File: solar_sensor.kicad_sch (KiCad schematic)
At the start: 4 parts

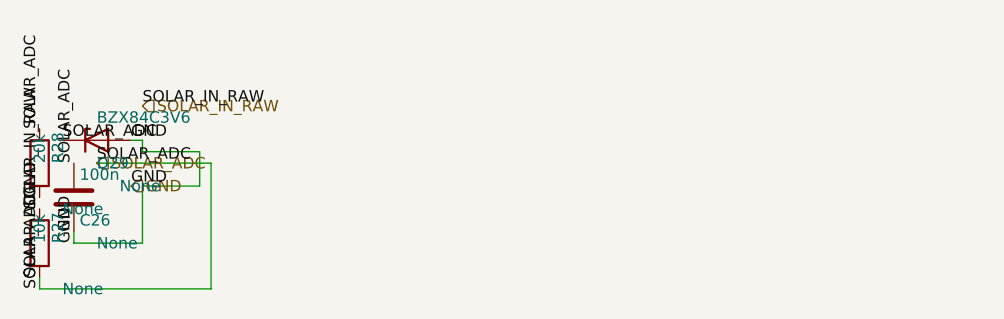
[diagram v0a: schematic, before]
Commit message: tests_fix
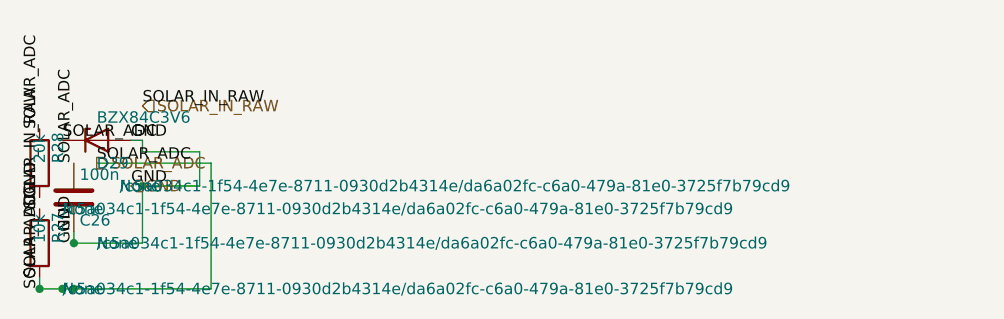
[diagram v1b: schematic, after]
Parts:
- C26, D29, R27, R28: hierarchy_path (none) -> /c5a034c1-1f54-4e7e-8711-0930d2b4314e/da6a02fc-c6a0-479a-81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
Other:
- title: (none) -> climate_control_niva_travel
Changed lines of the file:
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@@
 	(generator_version "9.0")
 	(paper "A4")
+	(title_block
+		(title "climate_control_niva_travel")
+	)
 	(symbol
 		(lib_id "Device:C")
@@
 			)
 		)
+		(property "hierarchy_path" "/c5a034c1-1f54-4e7e-8711-0930d2b4314e/da6a02fc-c6a0-479a-81e0-3725f7b79cd9"
+			(at 21.59 22.8599 0)
+			(effects
+				(font
+					(size 1.27 1.27)
+				)
+				(justify left)
+			)
+		)
 		(pin "1"
 		)
@@
 		)
 		(instances
-			(project "Untitled"
-				(path "/52be233a-28af-41aa-bdf8-43828795fcb1"
+			(project "climate_control_niva_travel"
+				(path "/c5a034c1-1f54-4e7e-8711-0930d2b4314e/da6a02fc-c6a0-479a-81e0-3725f7b79cd9"
 					(reference "C26")
 					(unit 1)
@@
 			)
 		)
+		(property "hierarchy_path" "/c5a034c1-1f54-4e7e-8711-0930d2b4314e/da6a02fc-c6a0-479a-81e0-3725f7b79cd9"
+			(at 17.78 27.9399 0)
+			(effects
+				(font
+					(size 1.27 1.27)
+				)
+				(justify left)
+			)
+		)
 		(pin "1"
 		)
@@
 		)
 		(instances
-			(project "Untitled"
-				(path "/52be233a-28af-41aa-bdf8-43828795fcb1"
-					(reference "R27")
+			(project "climate_control_niva_travel"
+				(path "/c5a034c1-1f54-4e7e-8711-0930d2b4314e/da6a02fc-c6a0-479a-81e0-3725f7b79cd9"
+					(reference "R43")
 					(unit 1)
 				)
@@
 			)
 		)
+		(property "hierarchy_path" "/c5a034c1-1f54-4e7e-8711-0930d2b4314e/da6a02fc-c6a0-479a-81e0-3725f7b79cd9"
+			(at 17.78 19.0499 0)
+			(effects
+				(font
+					(size 1.27 1.27)
+				)
+				(justify left)
+			)
+		)
 		(pin "1"
 		)
@@
 		)
 		(instances
-			(project "Untitled"
-				(path "/52be233a-28af-41aa-bdf8-43828795fcb1"
-					(reference "R28")
+			(project "climate_control_niva_travel"
+				(path "/c5a034c1-1f54-4e7e-8711-0930d2b4314e/da6a02fc-c6a0-479a-81e0-3725f7b79cd9"
+					(reference "R44")
 					(unit 1)
 				)
@@
 			)
 		)
+		(property "hierarchy_path" "/c5a034c1-1f54-4e7e-8711-0930d2b4314e/da6a02fc-c6a0-479a-81e0-3725f7b79cd9"
+			(at 24.13 16.5099 0)
+			(effects
+				(font
+					(size 1.27 1.27)
+				)
+				(justify left)
+			)
+		)
 		(pin "1"
 		)
@@
 		)
 		(instances
-			(project "Untitled"
-				(path "/52be233a-28af-41aa-bdf8-43828795fcb1"
+			(project "climate_control_niva_travel"
+				(path "/c5a034c1-1f54-4e7e-8711-0930d2b4314e/da6a02fc-c6a0-479a-81e0-3725f7b79cd9"
 					(reference "D29")
 					(unit 1)
@@
 			(type default)
 		)
+	)
+	(junction
+		(at 19.05 22.86)
+		(diameter 0)
+		(color 0 0 0 0)
+	)
+	(junction
+		(at 26.67 16.51)
+		(diameter 0)
+		(color 0 0 0 0)
+	)
+	(junction
+		(at 15.24 27.94)
+		(diameter 0)
+		(color 0 0 0 0)
+	)
+	(junction
+		(at 19.05 27.94)
+		(diameter 0)
+		(color 0 0 0 0)
+	)
+	(junction
+		(at 17.78 27.94)
+		(diameter 0)
+		(color 0 0 0 0)
 	)
 	(label "GND"
@@
 	)
 	(hierarchical_label "SOLAR_ADC"
-		(shape input)
+		(shape output)
 		(at 21.59 13.97 0)
 		(effects

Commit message: refactoring
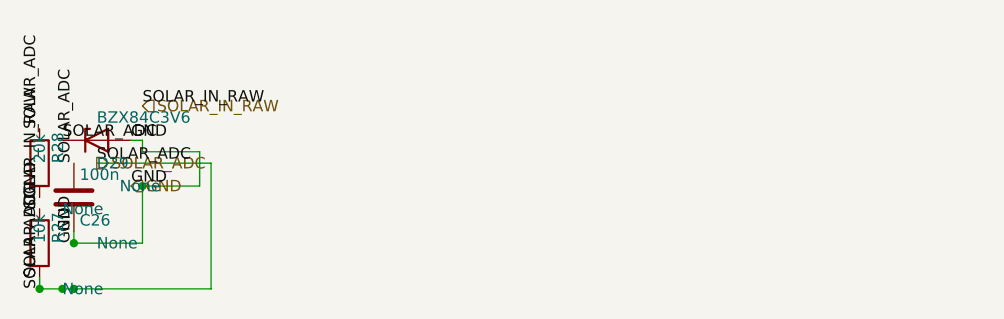
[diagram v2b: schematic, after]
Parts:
- C26, D29, R27, R28: hierarchy_path /c5a034c1-1f54-4e7e-8711-0930d2b4314e/da6a02fc-c6a0-479a-81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 -> (none)
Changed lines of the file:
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@@
-			)
-		)
-		(property "hierarchy_path" "/c5a034c1-1f54-4e7e-8711-0930d2b4314e/da6a02fc-c6a0-479a-81e0-3725f7b79cd9"
-			(at 21.59 22.8599 0)
-			(effects
-				(font
-					(size 1.27 1.27)
-				)
-				(justify left)
 			)
 		)
@@
 		(instances
 			(project "climate_control_niva_travel"
-				(path "/c5a034c1-1f54-4e7e-8711-0930d2b4314e/da6a02fc-c6a0-479a-81e0-3725f7b79cd9"
-					(reference "C26")
+				(path "/165a98f1-2dde-4141-9fdc-c935d39c8cff/bc23e0e1-20f6-4cfc-8f4c-1925d0779fcd/"
+					(reference "C0526")
 					(unit 1)
 				)
@@
 			)
 		)
-		(property "hierarchy_path" "/c5a034c1-1f54-4e7e-8711-0930d2b4314e/da6a02fc-c6a0-479a-81e0-3725f7b79cd9"
-			(at 17.78 27.9399 0)
-			(effects
-				(font
-					(size 1.27 1.27)
-				)
-				(justify left)
-			)
-		)
 		(pin "1"
 		)
@@
 		(instances
 			(project "climate_control_niva_travel"
-				(path "/c5a034c1-1f54-4e7e-8711-0930d2b4314e/da6a02fc-c6a0-479a-81e0-3725f7b79cd9"
-					(reference "R43")
+				(path "/165a98f1-2dde-4141-9fdc-c935d39c8cff/bc23e0e1-20f6-4cfc-8f4c-1925d0779fcd/"
+					(reference "R0527")
 					(unit 1)
 				)
@@
 			)
 		)
-		(property "hierarchy_path" "/c5a034c1-1f54-4e7e-8711-0930d2b4314e/da6a02fc-c6a0-479a-81e0-3725f7b79cd9"
-			(at 17.78 19.0499 0)
-			(effects
-				(font
-					(size 1.27 1.27)
-				)
-				(justify left)
-			)
-		)
 		(pin "1"
 		)
@@
 		(instances
 			(project "climate_control_niva_travel"
-				(path "/c5a034c1-1f54-4e7e-8711-0930d2b4314e/da6a02fc-c6a0-479a-81e0-3725f7b79cd9"
-					(reference "R44")
+				(path "/165a98f1-2dde-4141-9fdc-c935d39c8cff/bc23e0e1-20f6-4cfc-8f4c-1925d0779fcd/"
+					(reference "R0528")
 					(unit 1)
 				)
@@
 			)
 		)
-		(property "hierarchy_path" "/c5a034c1-1f54-4e7e-8711-0930d2b4314e/da6a02fc-c6a0-479a-81e0-3725f7b79cd9"
-			(at 24.13 16.5099 0)
-			(effects
-				(font
-					(size 1.27 1.27)
-				)
-				(justify left)
-			)
-		)
 		(pin "1"
 		)
@@
 		(instances
 			(project "climate_control_niva_travel"
-				(path "/c5a034c1-1f54-4e7e-8711-0930d2b4314e/da6a02fc-c6a0-479a-81e0-3725f7b79cd9"
-					(reference "D29")
+				(path "/165a98f1-2dde-4141-9fdc-c935d39c8cff/bc23e0e1-20f6-4cfc-8f4c-1925d0779fcd/"
+					(reference "D0529")
 					(unit 1)
 				)

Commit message: refactoring
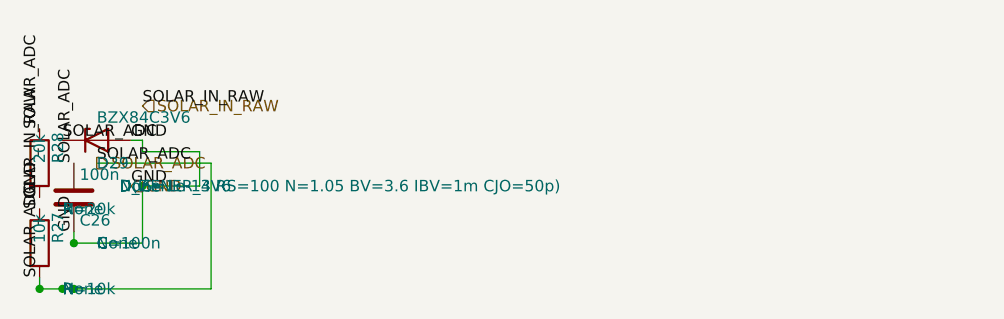
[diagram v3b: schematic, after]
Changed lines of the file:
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@@
+			)
+		)
+		(property "Sim.Device" "C"
+			(at 21.59 22.8599 0)
+			(effects
+				(font
+					(size 1.27 1.27)
+				)
+				(justify left)
+			)
+		)
+		(property "Sim.Params" "C=100n"
+			(at 21.59 22.8599 0)
+			(effects
+				(font
+					(size 1.27 1.27)
+				)
+				(justify left)
 			)
 		)
@@
 		(instances
 			(project "climate_control_niva_travel"
-				(path "/165a98f1-2dde-4141-9fdc-c935d39c8cff/bc23e0e1-20f6-4cfc-8f4c-1925d0779fcd/"
+				(path "/cc416b40-1361-4232-ac1e-5cd36ef0c0fb/0437e2fd-f00c-4872-bb50-cab86d166b22/"
 					(reference "C0526")
 					(unit 1)
@@
 			)
 		)
+		(property "Sim.Device" "R"
+			(at 17.78 27.9399 0)
+			(effects
+				(font
+					(size 1.27 1.27)
+				)
+				(justify left)
+			)
+		)
+		(property "Sim.Params" "R=10k"
+			(at 17.78 27.9399 0)
+			(effects
+				(font
+					(size 1.27 1.27)
+				)
+				(justify left)
+			)
+		)
 		(pin "1"
 		)
@@
 		(instances
 			(project "climate_control_niva_travel"
-				(path "/165a98f1-2dde-4141-9fdc-c935d39c8cff/bc23e0e1-20f6-4cfc-8f4c-1925d0779fcd/"
+				(path "/cc416b40-1361-4232-ac1e-5cd36ef0c0fb/0437e2fd-f00c-4872-bb50-cab86d166b22/"
 					(reference "R0527")
 					(unit 1)
@@
 			)
 		)
+		(property "Sim.Device" "R"
+			(at 17.78 19.0499 0)
+			(effects
+				(font
+					(size 1.27 1.27)
+				)
+				(justify left)
+			)
+		)
+		(property "Sim.Params" "R=20k"
+			(at 17.78 19.0499 0)
+			(effects
+				(font
+					(size 1.27 1.27)
+				)
+				(justify left)
+			)
+		)
 		(pin "1"
 		)
@@
 		(instances
 			(project "climate_control_niva_travel"
-				(path "/165a98f1-2dde-4141-9fdc-c935d39c8cff/bc23e0e1-20f6-4cfc-8f4c-1925d0779fcd/"
+				(path "/cc416b40-1361-4232-ac1e-5cd36ef0c0fb/0437e2fd-f00c-4872-bb50-cab86d166b22/"
 					(reference "R0528")
 					(unit 1)
@@
 			)
 		)
+		(property "Sim.Device" "D"
+			(at 24.13 16.5099 0)
+			(effects
+				(font
+					(size 1.27 1.27)
+				)
+				(justify left)
+			)
+		)
+		(property "Sim.Model" "D_ZENER_3V6"
+			(at 24.13 16.5099 0)
+			(effects
+				(font
+					(size 1.27 1.27)
+				)
+				(justify left)
+			)
+		)
+		(property "Sim.Params" "D(IS=1e-14 RS=100 N=1.05 BV=3.6 IBV=1m CJO=50p)"
+			(at 24.13 16.5099 0)
+			(effects
+				(font
+					(size 1.27 1.27)
+				)
+				(justify left)
+			)
+		)
 		(pin "1"
 		)
@@
 		(instances
 			(project "climate_control_niva_travel"
-				(path "/165a98f1-2dde-4141-9fdc-c935d39c8cff/bc23e0e1-20f6-4cfc-8f4c-1925d0779fcd/"
+				(path "/cc416b40-1361-4232-ac1e-5cd36ef0c0fb/0437e2fd-f00c-4872-bb50-cab86d166b22/"
 					(reference "D0529")
 					(unit 1)
@@
 	(junction
 		(at 19.05 22.86)
-		(diameter 0)
+		(diameter 0.0000)
 		(color 0 0 0 0)
 	)
 	(junction
 		(at 26.67 16.51)
-		(diameter 0)
+		(diameter 0.0000)
 		(color 0 0 0 0)
 	)
 	(junction
 		(at 15.24 27.94)
-		(diameter 0)
+		(diameter 0.0000)
 		(color 0 0 0 0)
 	)
 	(junction
 		(at 19.05 27.94)
-		(diameter 0)
+		(diameter 0.0000)
 		(color 0 0 0 0)
 	)
 	(junction
 		(at 17.78 27.94)
-		(diameter 0)
+		(diameter 0.0000)
 		(color 0 0 0 0)
 	)
@@
 		)
 	)
-	(label "GND"
-		(at 19.05 22.86 270)
-		(effects
-			(font
-				(size 1.27 1.27)
-			)
-			(justify left bottom)
-		)
-	)
 	(label "SOLAR_IN_RAW"
 		(at 15.24 19.05 90)
@@
 		(effects
 			(font
-				(size 1.27 1.27)
-			)
-			(justify left bottom)
-		)
-	)
-	(label "SOLAR_ADC"
-		(at 15.24 27.94 90)
-		(effects
-			(font
